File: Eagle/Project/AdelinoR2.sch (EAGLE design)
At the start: 79 parts, among them J1 DC-044-A, J2 YELLOW-8P-2.54, J3 YELLOW-6P-2.54, J4 YELLOW-8P-2.54, J5 YELLOW-8P-2.54, J6 4P-2.0, J7 YELLOW-2X3P-2.54, J8 4P-2.0, Q1 NCE3407A, Q2 CJ2305, SW1 TS-1101F, U1 CJT1117-3.3-SOT223, U2 MP1496DJ-SOT23-8, U3 ESP-12F / OPL: 317060163 / SM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, U4 ATMEGA32U4-MUR-QFN44, U5 ATMEGA32U4-TQFP44, X1 306010049_XTAL_16MHZ-3225_4P

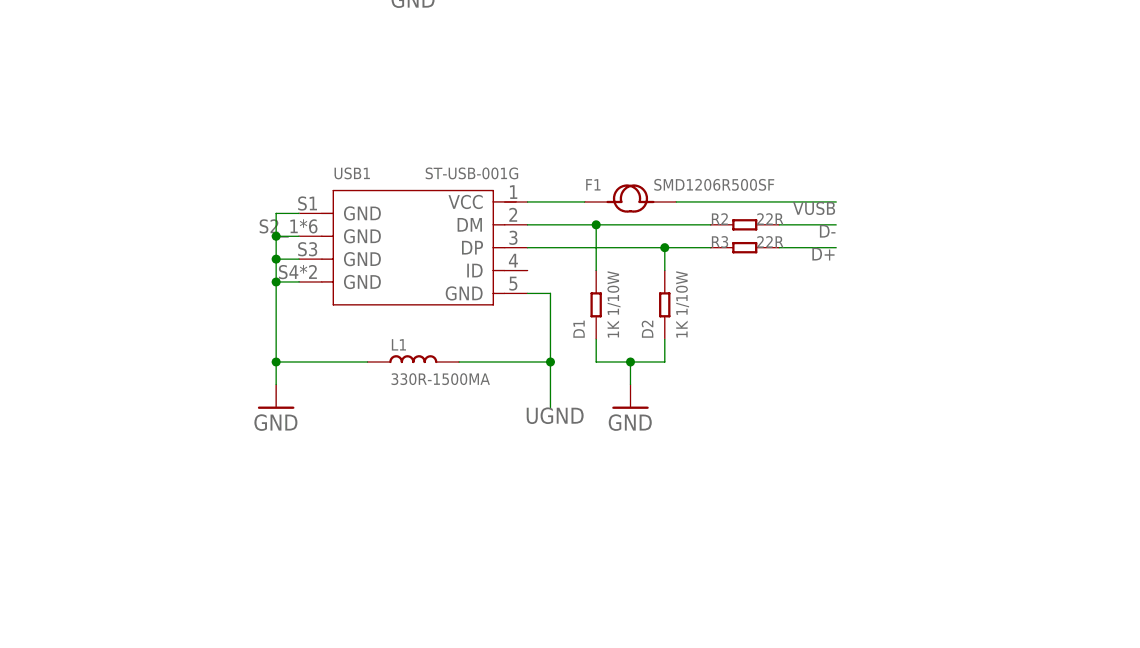
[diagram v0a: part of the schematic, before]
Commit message: Routing wip.
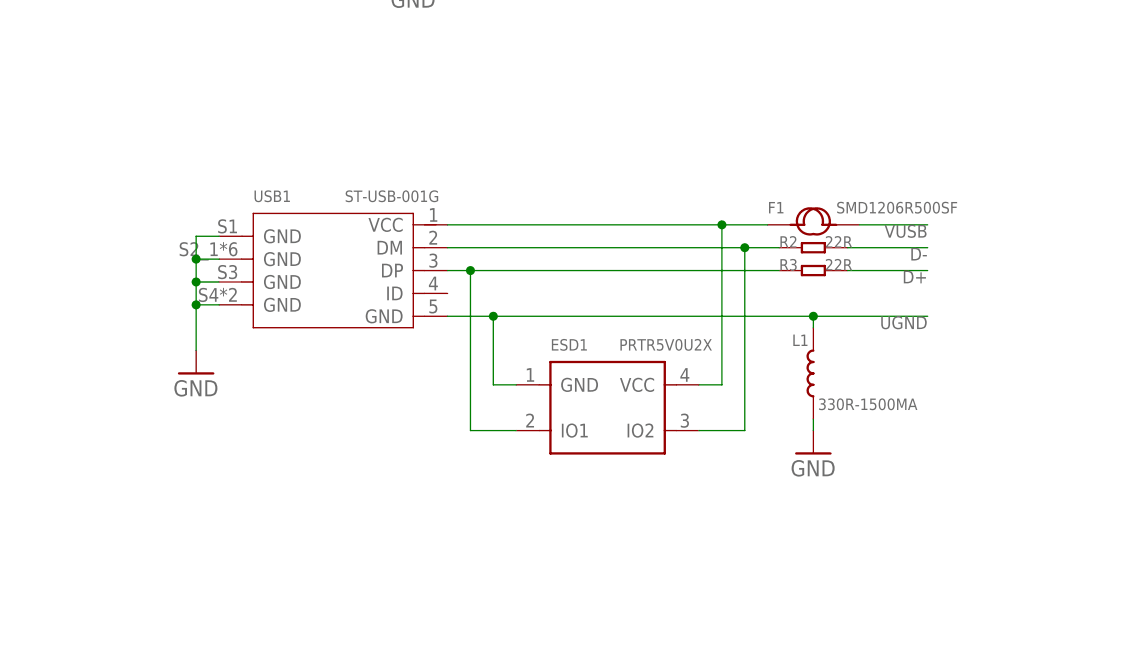
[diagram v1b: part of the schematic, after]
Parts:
- removed D1, D2: 1K 1/10W, Seeed-Fuse:SMD-ESD-CG0603MLC-05E
- added ESD1: PRTR5V0U2X, Seeed-OPL-2017-01-Diode-james:SMD-DIODE-TVS-5.5V
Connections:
- net GND: no longer D1.1, D2.1
- net N$1: now also ESD1.IO2; no longer D1.2
- net N$2: now also ESD1.IO1; no longer D2.2
- net N$9: now also ESD1.VCC
- net UGND: now also ESD1.GND
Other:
- moved on the sheet: F1, L1, R2, R3, USB1
